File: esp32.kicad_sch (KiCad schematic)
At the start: 5 parts, among them U2 ESP32-S3-WROOM-1

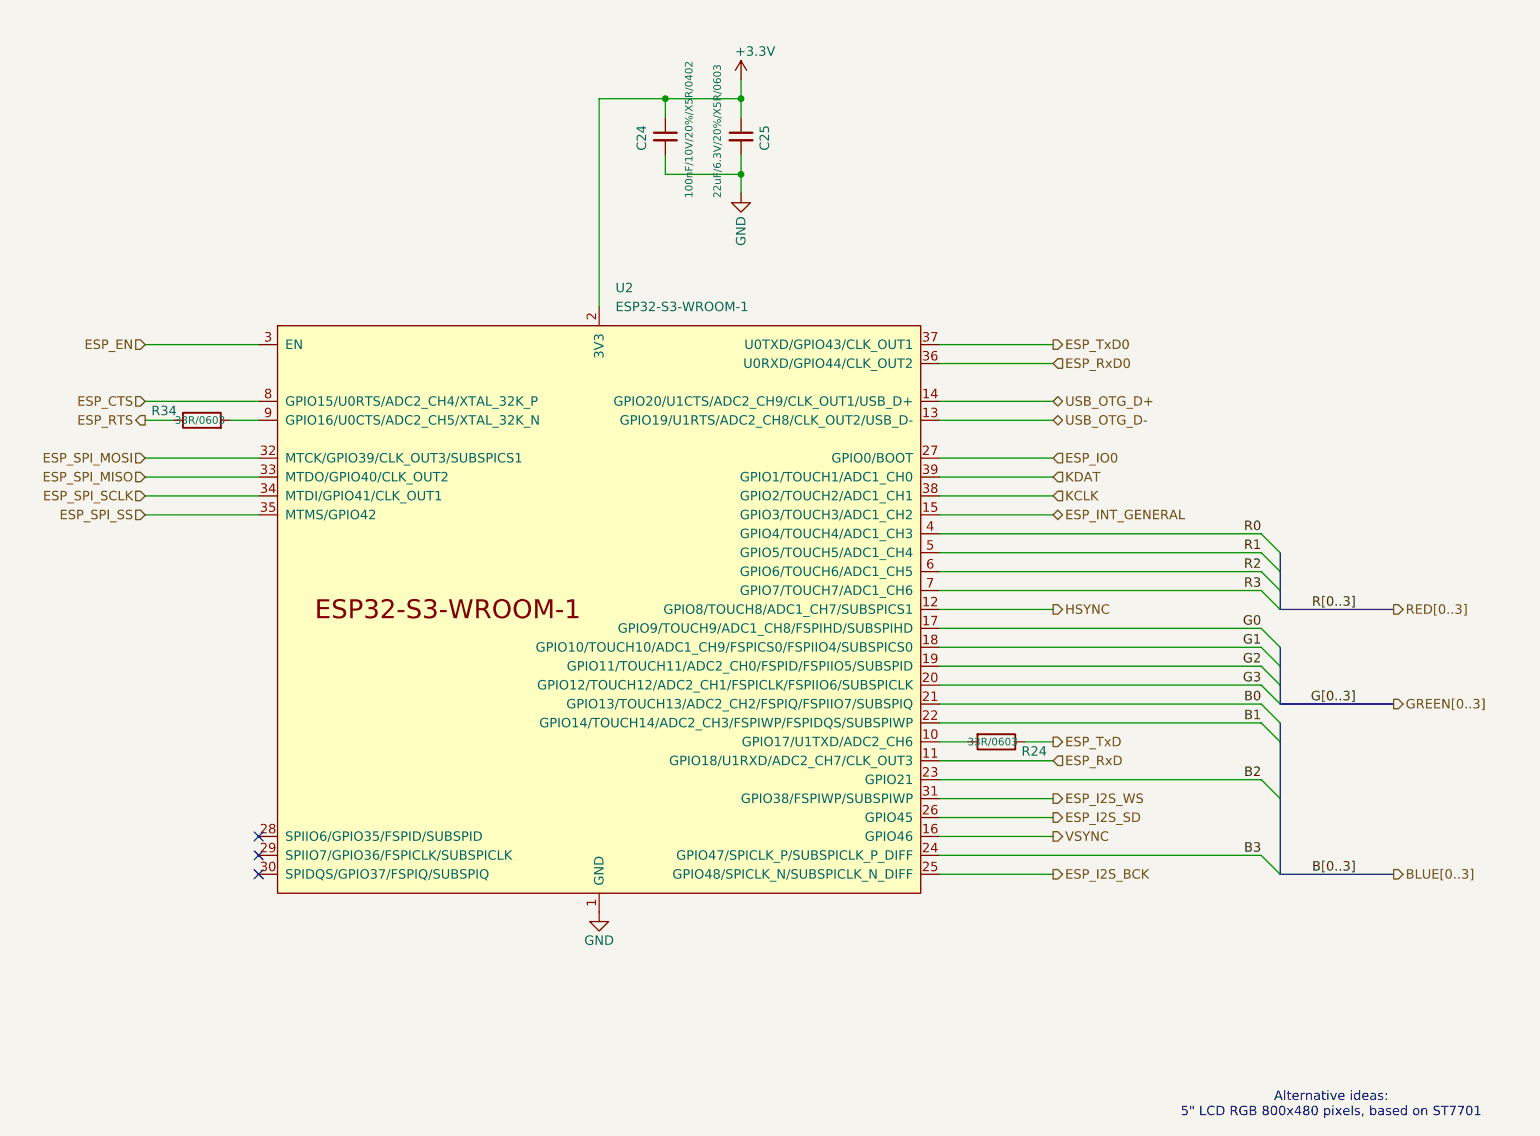
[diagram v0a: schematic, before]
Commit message: 1st production and BOM
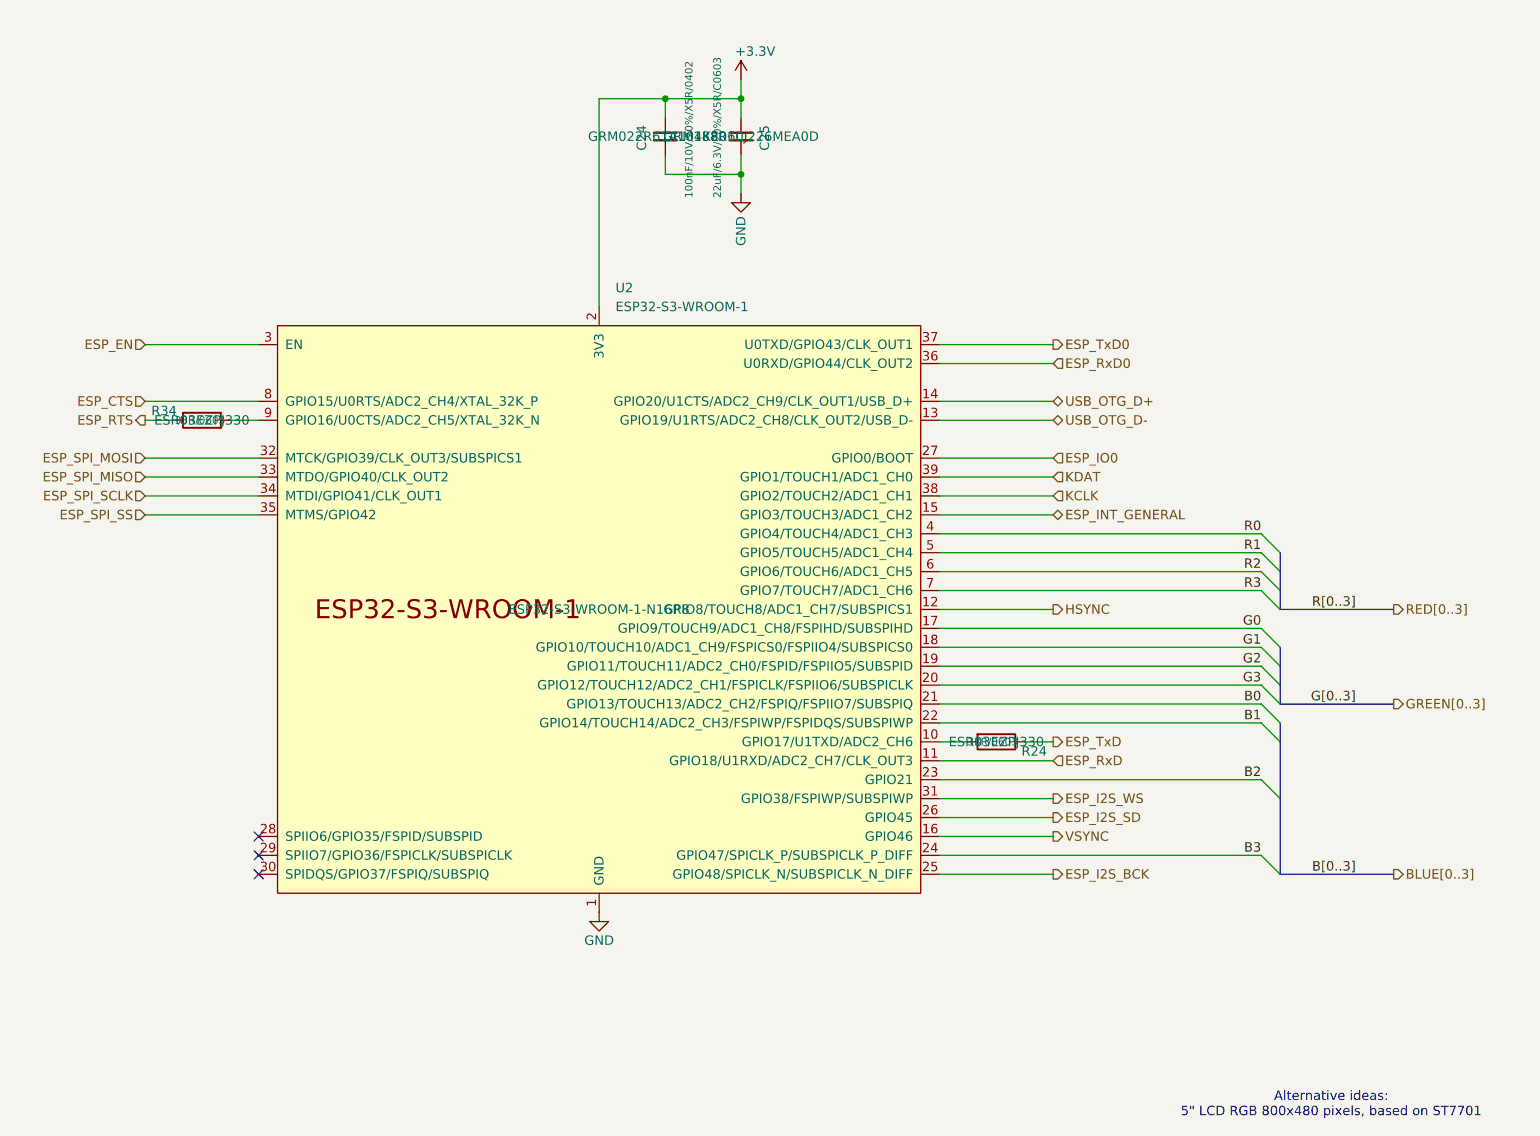
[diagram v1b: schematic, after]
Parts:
- C24: MfgNumber (none) -> GRM022R61A104KE01L
- C25: value 22uF/6.3V/20%/X5R/0603 -> 22uF/6.3V/20%/X5R/C0603; MfgNumber (none) -> GRM188R60J226MEA0D
- R24, R34: MfgNumber (none) -> ESR03EZPJ330
- U2: MfgNumber (none) -> ESP32-S3-WROOM-1-N16R8
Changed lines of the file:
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@@
 			)
 		)
-		(property "Value" "22uF/6.3V/20%/X5R/0603"
+		(property "Value" "22uF/6.3V/20%/X5R/C0603"
 			(at 150.495 52.705 90)
 			(effects
@@
 				)
 				(hide yes)
+			)
+		)
+		(property "Note" ""
+			(at 153.67 44.45 0)
+			(effects
+				(font
+					(size 1.27 1.27)
+				)
+			)
+		)
+		(property "MfgNumber" "GRM188R60J226MEA0D"
+			(at 153.67 44.45 0)
+			(effects
+				(font
+					(size 1.27 1.27)
+				)
 			)
 		)
@@
 			)
 		)
+		(property "Note" ""
+			(at 143.51 44.45 0)
+			(effects
+				(font
+					(size 1.27 1.27)
+				)
+			)
+		)
+		(property "MfgNumber" "GRM022R61A104KE01L"
+			(at 143.51 44.45 0)
+			(effects
+				(font
+					(size 1.27 1.27)
+				)
+			)
+		)
 		(pin "1"
 		)
@@
 				)
 				(hide yes)
+			)
+		)
+		(property "Note" ""
+			(at 81.28 82.55 0)
+			(effects
+				(font
+					(size 1.27 1.27)
+				)
+			)
+		)
+		(property "MfgNumber" "ESR03EZPJ330"
+			(at 81.28 82.55 0)
+			(effects
+				(font
+					(size 1.27 1.27)
+				)
 			)
 		)
@@
 			)
 		)
+		(property "Note" ""
+			(at 134.62 107.95 0)
+			(effects
+				(font
+					(size 1.27 1.27)
+				)
+			)
+		)
+		(property "MfgNumber" "ESP32-S3-WROOM-1-N16R8"
+			(at 134.62 107.95 0)
+			(effects
+				(font
+					(size 1.27 1.27)
+				)
+			)
+		)
 		(pin "27"
 		)
@@
 			)
 		)
+		(property "Note" ""
+			(at 187.96 125.73 0)
+			(effects
+				(font
+					(size 1.27 1.27)
+				)
+			)
+		)
+		(property "MfgNumber" "ESR03EZPJ330"
+			(at 187.96 125.73 0)
+			(effects
+				(font
+					(size 1.27 1.27)
+				)
+			)
+		)
